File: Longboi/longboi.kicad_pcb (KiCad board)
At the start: 2 copper layers, 383 x 78.2 mm, 200 parts, among them J2 ICSP_Header, K0 KEYSW, K1 KEYSW, K10 KEYSW, K11 KEYSW, K12 KEYSW, K13 KEYSW, K14 KEYSW, K15 KEYSW, K16 KEYSW, K17 KEYSW, K18 KEYSW, K19 KEYSW, K2 KEYSW, K20 KEYSW, K21 KEYSW, K22 KEYSW, K22-spacer1 KEYSW, K22-stepped1 KEYSW, K23 KEYSW, K24 KEYSW, K25 KEYSW, K26 KEYSW, K27 KEYSW, K28 KEYSW, K29 KEYSW, K3 KEYSW, K3-2uVert1 KEYSW, K30 KEYSW, K31 KEYSW, K32 KEYSW, K33 KEYSW, K34 KEYSW, K35 KEYSW, K36 KEYSW, K37 KEYSW, K38 KEYSW, K38-2uVert1 KEYSW, K39 KEYSW, K39-spacer1 KEYSW, K4 KEYSW, K4-spacer1 KEYSW, K40 KEYSW, K41 KEYSW, K42 KEYSW, K43 KEYSW, K44 KEYSW, K45 KEYSW, K46 KEYSW, K47 KEYSW, K48 KEYSW, K49 KEYSW, K5 KEYSW, K50 KEYSW, K51 KEYSW, K52 KEYSW, K52-1u1 KEYSW, K52-2u1 KEYSW, K53 KEYSW, K54 KEYSW, K55 KEYSW, K55-1.25 KEYSW, K55-spacer1 KEYSW, K55-spacer2 KEYSW, K56 KEYSW, K56-1.25 KEYSW, K57 KEYSW, K57-1.25 KEYSW, K57-1.5u1 KEYSW, K57-1u1 KEYSW, K58 KEYSW, K58-6u1 KEYSW, K58for1.25Row1 KEYSW, K59 KEYSW, K59-1.25u1 KEYSW, K59-7u1 KEYSW, K59Alt1 KEYSW, K6 KEYSW, K60 KEYSW, K60Alt1 KEYSW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

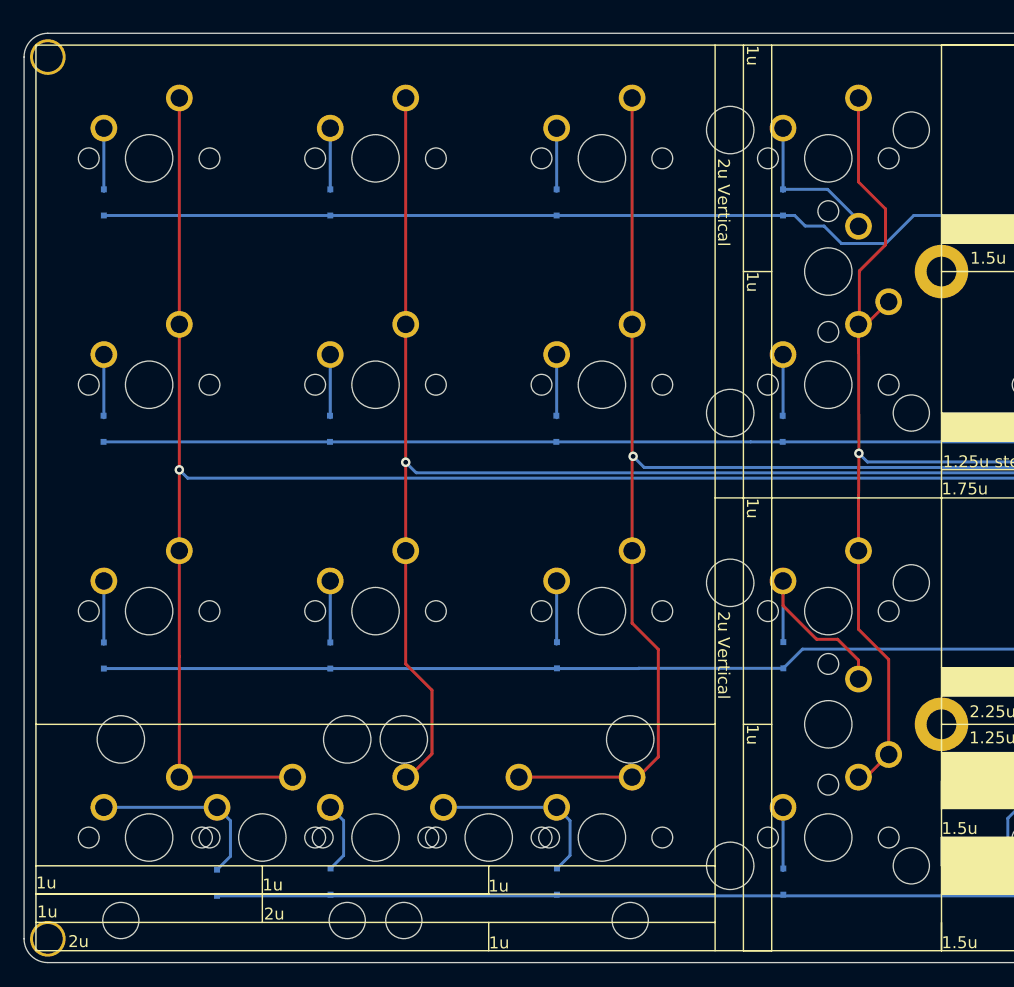
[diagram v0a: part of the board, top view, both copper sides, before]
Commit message: moreupdates to tweak the two keyboards
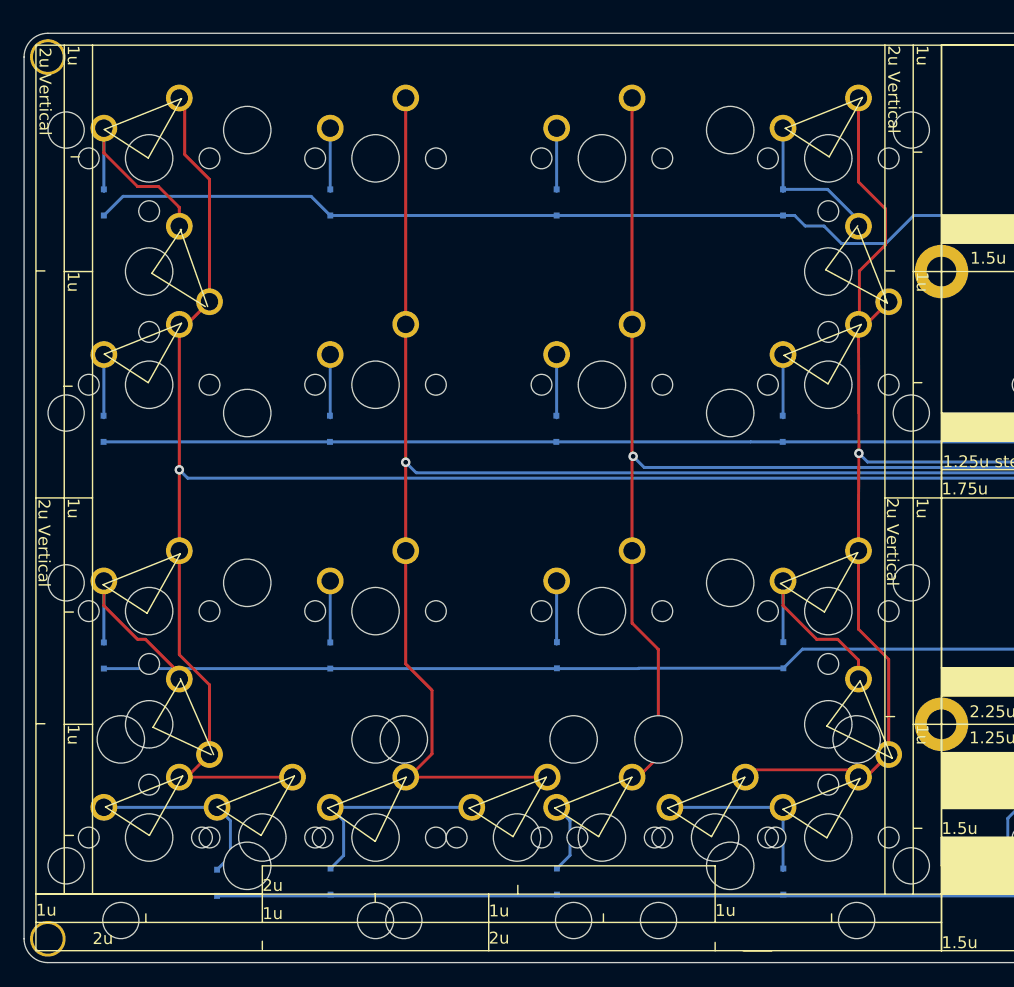
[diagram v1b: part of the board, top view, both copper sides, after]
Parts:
- removed K52-2u1: KEYSW, MX_Only:MXOnly-2U-ReversedStabilizers-NoLED
- added K0-2uVert1: KEYSW, MX_Only:MXOnly-2U-ReversedStabilizers-NoLED, F.Cu at (25.3, 39.4)
- added K35-2uVert1: KEYSW, MX_Only:MXOnly-2U-ReversedStabilizers-NoLED, F.Cu at (25.3, 77.5)
- added K54-2u1: KEYSW, MX_Only:MXOnly-2U-ReversedStabilizers-NoLED, F.Cu at (72.9, 87.0)
- added K70-2u1: KEYSW, MX_Only:MXOnly-2U-ReversedStabilizers-NoLED, F.Cu at (56.2, 87.0)
- moved Ge 62.0 mm to (98.3, 66.5)
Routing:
- net Net-(D0-Pad2): track 5.33 -> 17.2 mm
- net Net-(D70-Pad2): track 6.07 -> 18.0 mm
- net /Col_1: track 342.1 -> 354.0 mm
- net Net-(D35-Pad2): track 5.33 -> 16.6 mm
- net /Col_3: track 309.5 -> 319.5 mm
- net Net-(D53-Pad2): track 15.6 -> 6.07 mm
- net /Col_2: track 332.5 -> 323.0 mm
- net Net-(D54-Pad2): track 5.33 -> 14.8 mm
- net /Col_0: track 368.4 -> 373.6 mm
- net /Row_0: track 399.9 -> 401.2 mm
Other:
- board text added: "MountingHole"
